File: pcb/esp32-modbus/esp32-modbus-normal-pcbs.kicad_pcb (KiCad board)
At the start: 2 copper layers, 85.8 x 77.9 mm, 54 parts, among them J1 Conn_01x01_Male, J10 Conn_01x01_Male, J12 Conn_01x01_Male, J13 Conn_01x01_Male, J2 Conn_01x05_Male, J22 Conn_01x01_Male, J23 Conn_01x01_Male, J24 Conn_01x01_Male, J25 Conn_01x01_Male, J26 Conn_01x01_Male, J27_VCC1 Conn_01x01_Male, J28_RO1 Conn_01x01_Male, J29_DI1 Conn_01x01_Male, J3 Conn_01x01_Male, J30_RE/DE1 Conn_01x01_Male, J31_GND1 Conn_01x01_Male, J4 Conn_01x01_Male, J5 Conn_01x01_Male, J6 Screw_Terminal_01x02, J7 Conn_01x09_Male, J8 Conn_01x09_Male, J9 Conn_01x01_Male, Q1 BC817, Q2 BC817, U1 ESP32-WROOM-32U

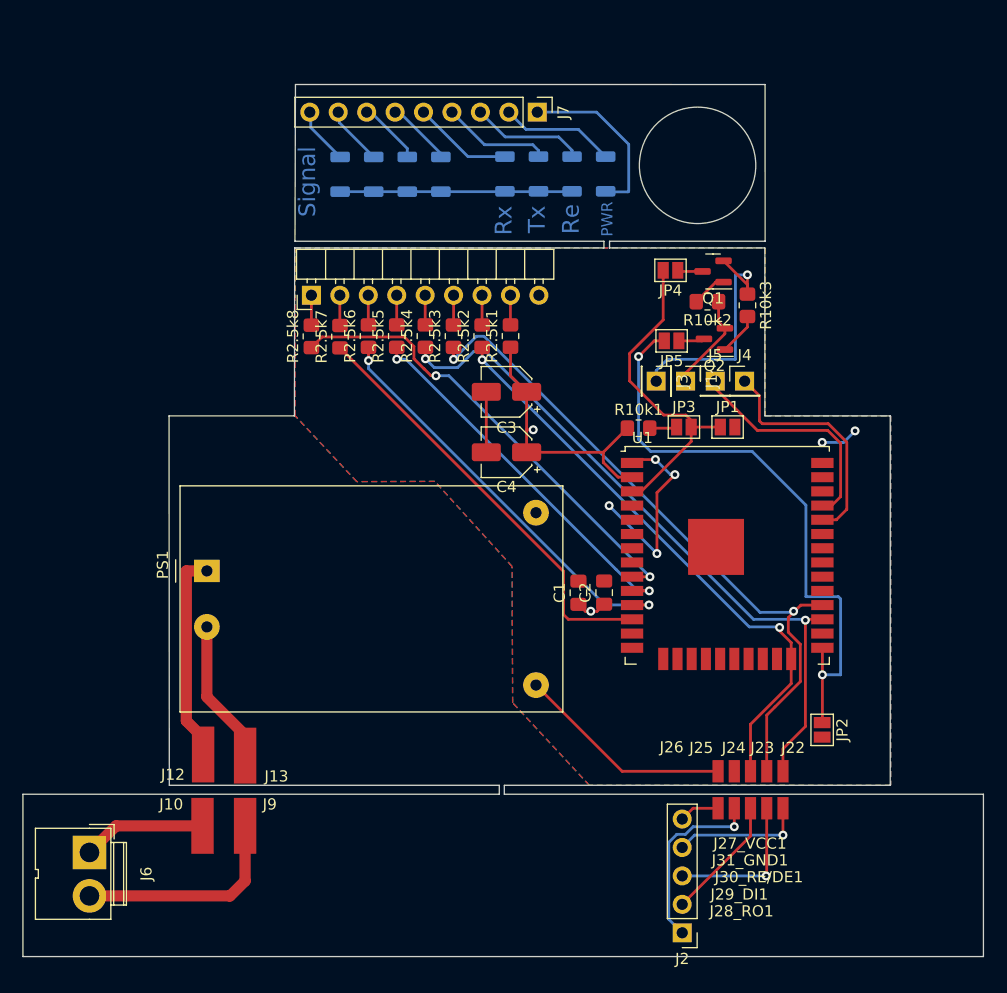
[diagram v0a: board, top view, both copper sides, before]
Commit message: full prototype
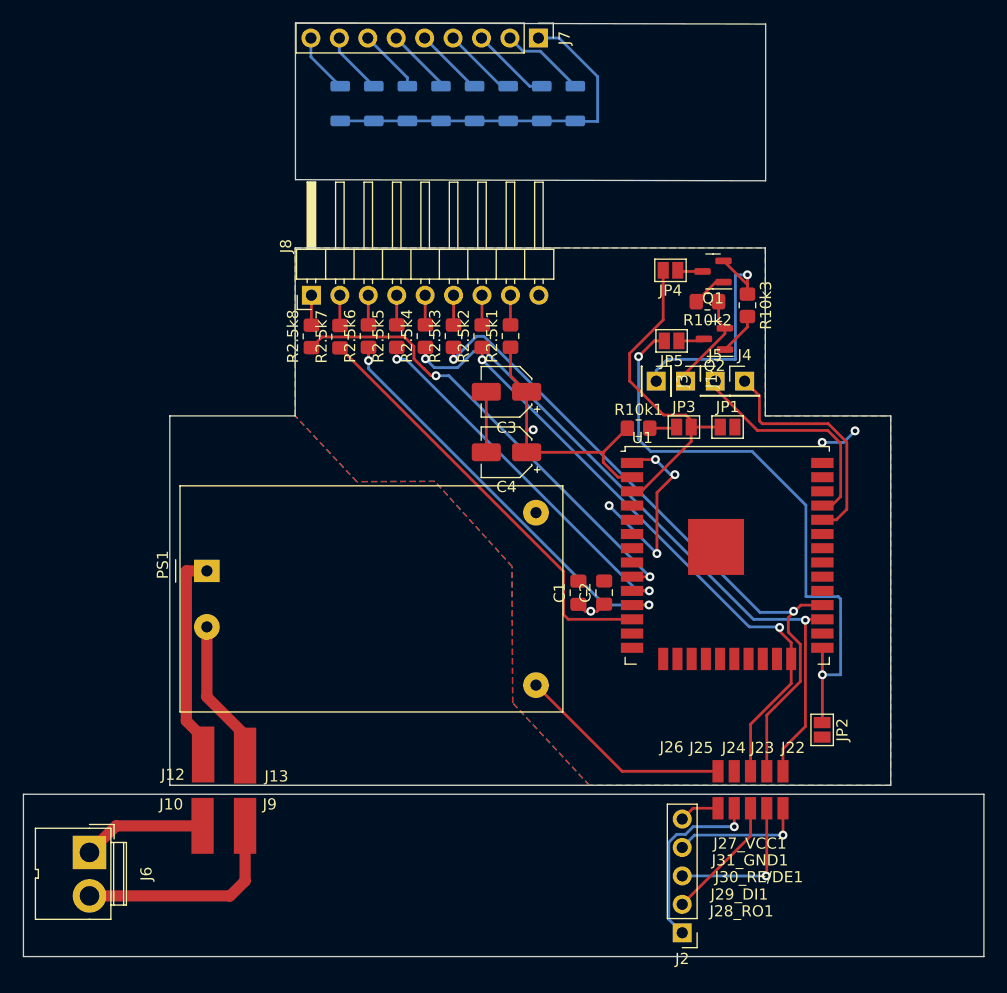
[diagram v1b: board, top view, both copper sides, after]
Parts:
- moved D1 6.85 mm to (175.2, 71.4)
- moved D2 6.85 mm to (172.2, 71.4)
- moved D3 6.85 mm to (169.2, 71.4)
- moved D4 6.85 mm to (178.2, 71.4)
- moved J7 6.62 mm to (174.9, 65.5)
- moved D5 6.32 mm to (166.2, 71.4)
- moved D6 6.32 mm to (163.2, 71.4)
- moved D7 6.32 mm to (160.2, 71.4)
- moved D8 6.32 mm to (157.2, 71.4)
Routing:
- net Net-(D2-Pad2): track 10.3 -> 6.70 mm
- net Net-(D1-Pad2): track 10.2 -> 7.16 mm
- net Net-(D1-Pad1): track 36.7 -> 33.7 mm
- net Net-(D4-Pad2): track 10.3 -> 7.62 mm
- net Net-(D3-Pad2): track 8.91 -> 6.24 mm
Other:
- board size 85.8 x 77.9 mm -> 85.8 x 83.4 mm
- board text removed: "PWR"
- board text removed: "Re"
- board text removed: "Rx"
- board text removed: "Signal"
- board text removed: "Tx"
